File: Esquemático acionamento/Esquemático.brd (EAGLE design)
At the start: 101.3 x 44.4 mm, 9 parts

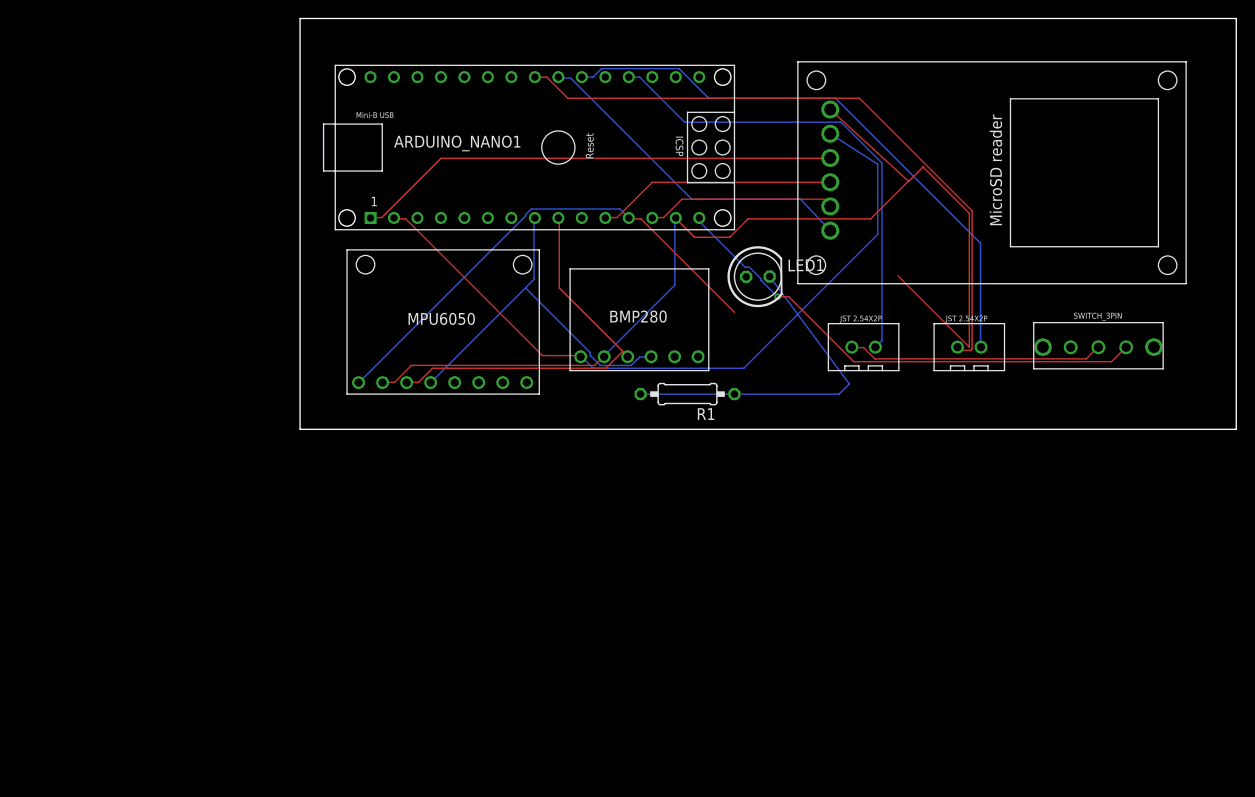
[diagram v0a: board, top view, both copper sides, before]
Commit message: Update
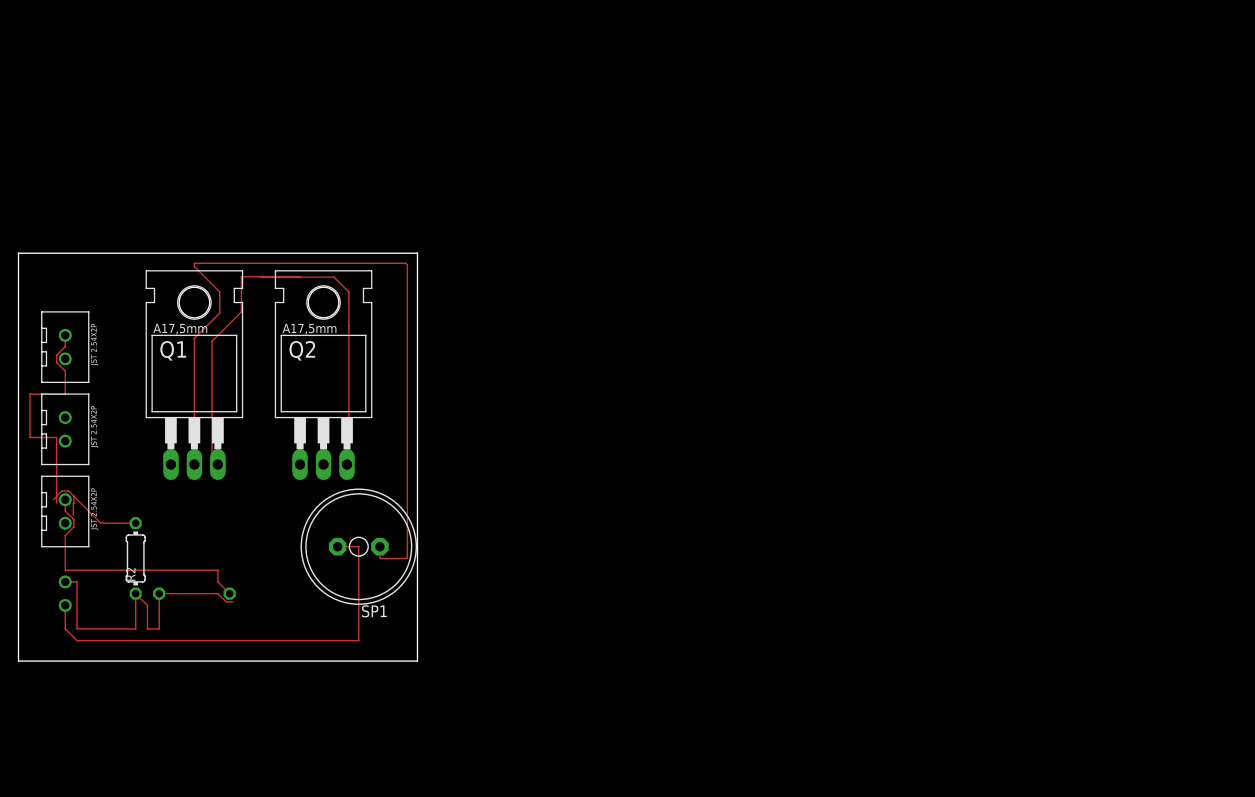
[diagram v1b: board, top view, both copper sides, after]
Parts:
- removed ARDUINO_NANO1: (no value), ArduinoNanoV30:ARDUINO_NANO
- removed LED1: (no value), led:LED5MM
- removed U$5, U$6: JST2.54X2P, CRD:JST2.54X2P_FOOTPRINT
- added Q1, Q2: IRF540, transistor-fet:TO220
- added R2: 1k, rcl:0204/7
- added SP1: AL11P, buzzer:AL11P
- R1: value (none) -> 1k; device rcl:0207/10 -> rcl:0204/7
- U$1: value BMP280V1 -> JST2.54X2P; device CRD:BMP280_FOOTPRINT -> CRD:JST2.54X2P_FOOTPRINT
- U$2: value MPU6050V1 -> JST2.54X2P; device CRD:MPU6050_FOOTPRINT -> CRD:JST2.54X2P_FOOTPRINT
- U$3: value MICROSD_READER -> JST2.54X2P; device CRD:MICROSD_READER_FOOTPRINT -> CRD:JST2.54X2P_FOOTPRINT
- U$4: value SWITCH_3PIN -> JST2.54X2P; device CRD:SWITCH_3PIN -> CRD:JST2.54X2P_FOOTPRINT
- moved U$4 114.9 mm to (-25.4, -17.8), flipped to the bottom, turned to 90 degrees
- moved U$3 93.4 mm to (-25.4, 8.89)
- moved U$1 66.3 mm to (-25.4, -8.89), turned to 270 degrees
- moved R1 57.5 mm to (-11.4, -17.8), flipped to the bottom
- moved U$2 43.4 mm to (-25.4, 0.00), turned to 270 degrees
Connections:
- removed net N$10: LED1.K, R1.2
- removed net N$11: ARDUINO_NANO1.21, LED1.A, U$5.2
- removed net N$12: ARDUINO_NANO1.19, U$6.2
- removed net N$13: ARDUINO_NANO1.23, U$5.1
- removed net N$14: ARDUINO_NANO1.15, U$4.3
- removed net N$15: U$4.2, U$6.1
- removed net N$6: ARDUINO_NANO1.22, U$3.CS
- removed net N$7: ARDUINO_NANO1.13, U$3.SCK
- removed net N$8: ARDUINO_NANO1.11, U$3.MOSI
- removed net N$9: ARDUINO_NANO1.1, U$3.MISO
- new net 0: Q1.3, Q2.3, R1.1, R2.1, U$4.2
- new net VCC: SP1.+, U$4.1
- net N$1: now also Q2.1, R1.2, U$1.1; no longer ARDUINO_NANO1.2, U$1.VCC, U$3.VCC
- net N$2: now also Q2.2, U$2.2; no longer ARDUINO_NANO1.9, U$1.SCL, U$2.SCL
- net N$3: now also Q1.1, R2.2, U$3.1; no longer ARDUINO_NANO1.8, U$1.SDA, U$2.SDA
- net N$4: now also U$2.1; no longer ARDUINO_NANO1.14, R1.1, U$1.GND, U$2.GND, U$3.GND
- net N$5: now also Q1.2, SP1.-; no longer ARDUINO_NANO1.12, U$2.VCC
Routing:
- net N$4: track 118.1 -> 0.00 mm
- net 0: track 0.00 -> 91.5 mm
- net N$13: track 70.0 -> 0.00 mm
- net N$11: track 62.6 -> 0.00 mm
- net N$14: track 53.6 -> 0.00 mm, vias 1 -> 0
- net N$9: track 52.4 -> 0.00 mm
- net N$12: track 51.4 -> 0.00 mm
- net N$1: track 78.8 -> 28.0 mm
- net VCC: track 0.00 -> 47.3 mm
- net N$2: track 42.9 -> 0.19 mm
- net N$10: track 37.5 -> 0.00 mm
- net N$6: track 36.3 -> 0.00 mm
- net N$5: track 53.2 -> 83.1 mm
- net N$15: track 27.7 -> 0.00 mm
- net N$8: track 25.9 -> 0.00 mm
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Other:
- board size 101.3 x 44.4 mm -> 43.2 x 44.1 mm

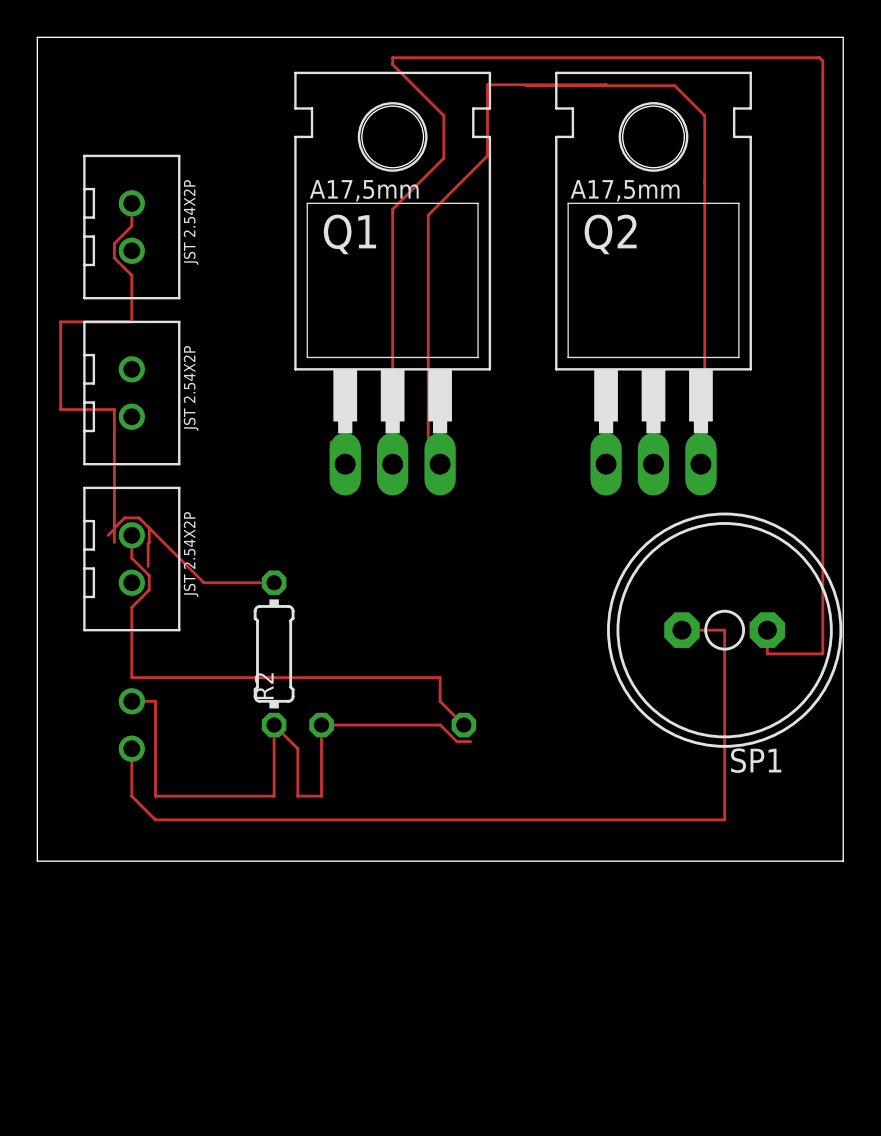
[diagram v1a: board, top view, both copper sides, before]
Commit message: Add files via upload
Placa de Acionamento
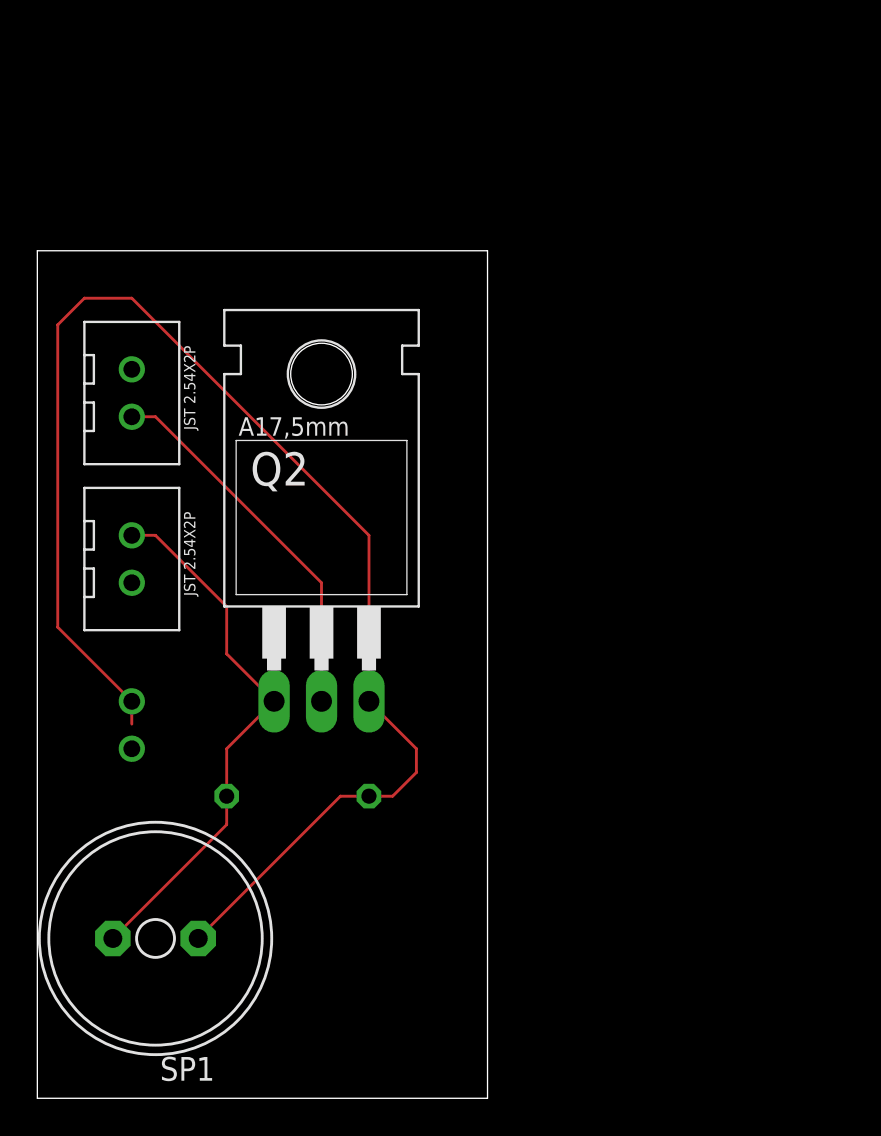
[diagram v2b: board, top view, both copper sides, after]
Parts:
- removed Q1: IRF540, transistor-fet:TO220
- removed R2: 1k, rcl:0204/7
- removed U$3: JST2.54X2P, CRD:JST2.54X2P_FOOTPRINT
- moved SP1 34.7 mm to (-24.1, -29.2)
- moved Q2 21.8 mm to (-15.2, -10.2)
- moved R1 6.35 mm to (-16.5, -21.6), turned to 0 degrees
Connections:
- removed net N$3: Q1.1, R2.2, U$3.1
- removed net N$5: Q1.2, SP1.-
- net 0: now also SP1.-; no longer Q1.3, R2.1
- net N$1: now also SP1.+
- net VCC: no longer SP1.+
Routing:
- net N$5: track 83.1 -> 0.00 mm
- net VCC: track 47.3 -> 0.00 mm
- net N$3: track 38.9 -> 0.00 mm
- net N$2: track 0.19 -> 20.4 mm
- net 0: track 91.5 -> 76.5 mm
- net N$1: track 28.0 -> 29.1 mm
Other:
- board size 43.2 x 44.1 mm -> 24.1 x 45.4 mm
